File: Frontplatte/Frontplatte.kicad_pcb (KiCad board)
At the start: 2 copper layers, 49 parts, among them J1 Conn_01x04_Male, J2 Conn_01x04_Male, J3 Conn_01x04_Male, J4 Conn_01x04_Male, J5 Conn_01x04_Male, SW1 SW_DIP_x04, U1 MCP23017_SP

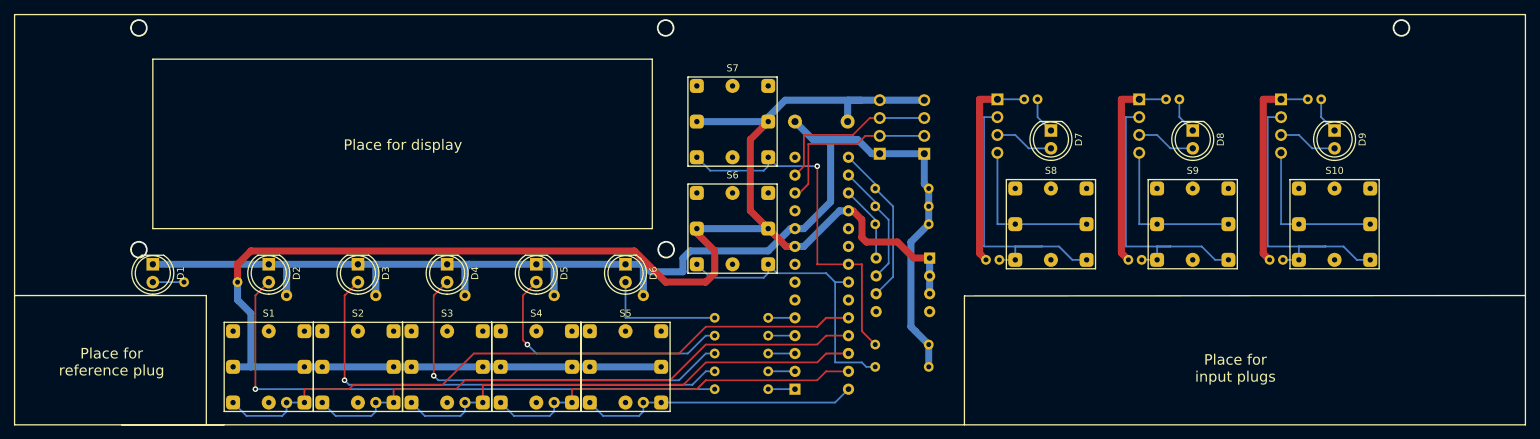
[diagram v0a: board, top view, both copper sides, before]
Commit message: Updated
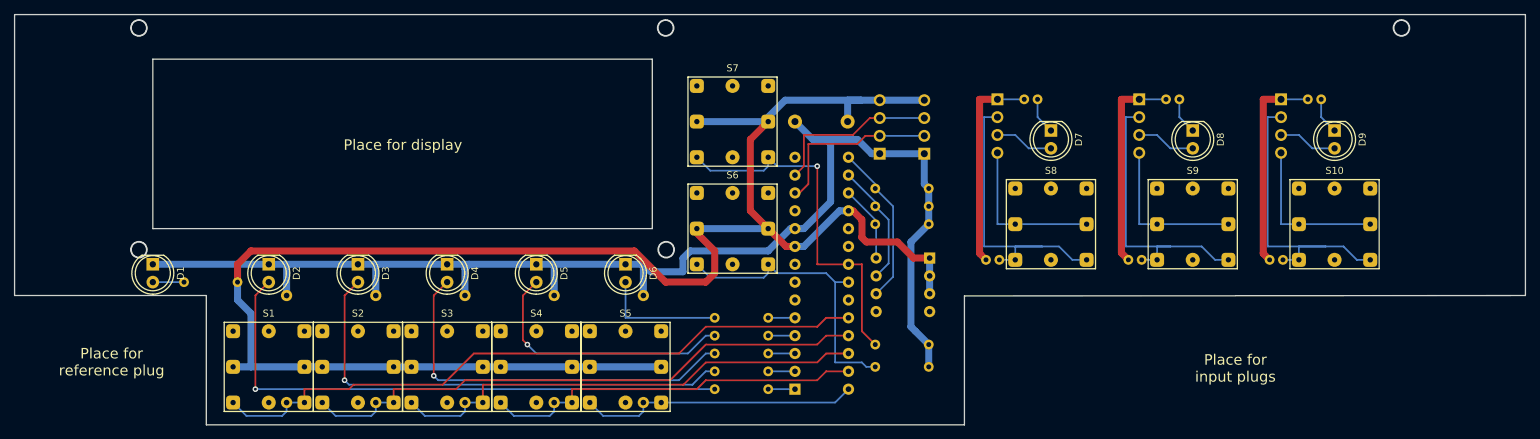
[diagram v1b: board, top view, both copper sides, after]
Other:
- board outline added: 215.1 x 58.4 mm
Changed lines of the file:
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@@
     )
   )
-  (gr_line (start 34.925 102.235) (end 34.925 43.815) (layer "F.SilkS") (width 0.15))
-  (gr_line (start 54.61 50.165) (end 54.61 74.295) (layer "F.SilkS") (width 0.15))
-  (gr_line (start 125.73 74.295) (end 125.73 50.165) (layer "F.SilkS") (width 0.15))
-  (gr_line (start 64.77 102.235) (end 34.925 102.235) (layer "F.SilkS") (width 0.15))
-  (gr_line (start 250.063 102.235) (end 50.165 102.235) (layer "F.SilkS") (width 0.15))
-  (gr_line (start 170.18 83.8835) (end 170.18 102.235) (layer "F.SilkS") (width 0.15))
-  (gr_line (start 125.73 50.165) (end 54.61 50.165) (layer "F.SilkS") (width 0.15))
-  (gr_line (start 34.925 43.815) (end 250.063 43.815) (layer "F.SilkS") (width 0.15))
-  (gr_line (start 34.925 83.82) (end 62.23 83.82) (layer "F.SilkS") (width 0.15))
-  (gr_line (start 62.23 83.82) (end 62.23 102.235) (layer "F.SilkS") (width 0.15))
-  (gr_line (start 250.063 83.82) (end 170.18 83.8835) (layer "F.SilkS") (width 0.15))
-  (gr_line (start 54.61 74.295) (end 125.73 74.295) (layer "F.SilkS") (width 0.15))
-  (gr_line (start 250.063 43.815) (end 250.063 102.235) (layer "F.SilkS") (width 0.15))
+  (gr_line (start 34.925 83.82) (end 34.925 43.815) (layer "Edge.Cuts") (width 0.15))
+  (gr_line (start 54.61 50.165) (end 54.61 74.295) (layer "Edge.Cuts") (width 0.15))
+  (gr_line (start 125.73 74.295) (end 125.73 50.165) (layer "Edge.Cuts") (width 0.15))
+  (gr_line (start 170.18 102.235) (end 62.23 102.235) (layer "Edge.Cuts") (width 0.15))
+  (gr_line (start 170.18 83.8835) (end 170.18 102.235) (layer "Edge.Cuts") (width 0.15))
+  (gr_line (start 125.73 50.165) (end 54.61 50.165) (layer "Edge.Cuts") (width 0.15))
+  (gr_line (start 34.925 43.815) (end 250.063 43.815) (layer "Edge.Cuts") (width 0.15))
+  (gr_line (start 34.925 83.82) (end 62.23 83.82) (layer "Edge.Cuts") (width 0.15))
+  (gr_line (start 62.23 83.82) (end 62.23 102.235) (layer "Edge.Cuts") (width 0.15))
+  (gr_line (start 250.063 83.82) (end 170.18 83.8835) (layer "Edge.Cuts") (width 0.15))
+  (gr_line (start 54.61 74.295) (end 125.73 74.295) (layer "Edge.Cuts") (width 0.15))
+  (gr_line (start 250.063 43.815) (end 250.063 83.82) (layer "Edge.Cuts") (width 0.15))
   (gr_text "VCC" (at 161.29 56.007) (layer "B.SilkS")
     (effects (font (size 1 1) (thickness 0.15)) (justify mirror))
